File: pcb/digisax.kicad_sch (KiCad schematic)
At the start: 53 parts, among them SW1 RotaryEncoder_Switch, U1 ER_OLEDM0.91_1x-I2C, U2 MPXV7007, U3 MCP3221, U4 TLV320DAC3100_breakout, U5 ESP32-S3

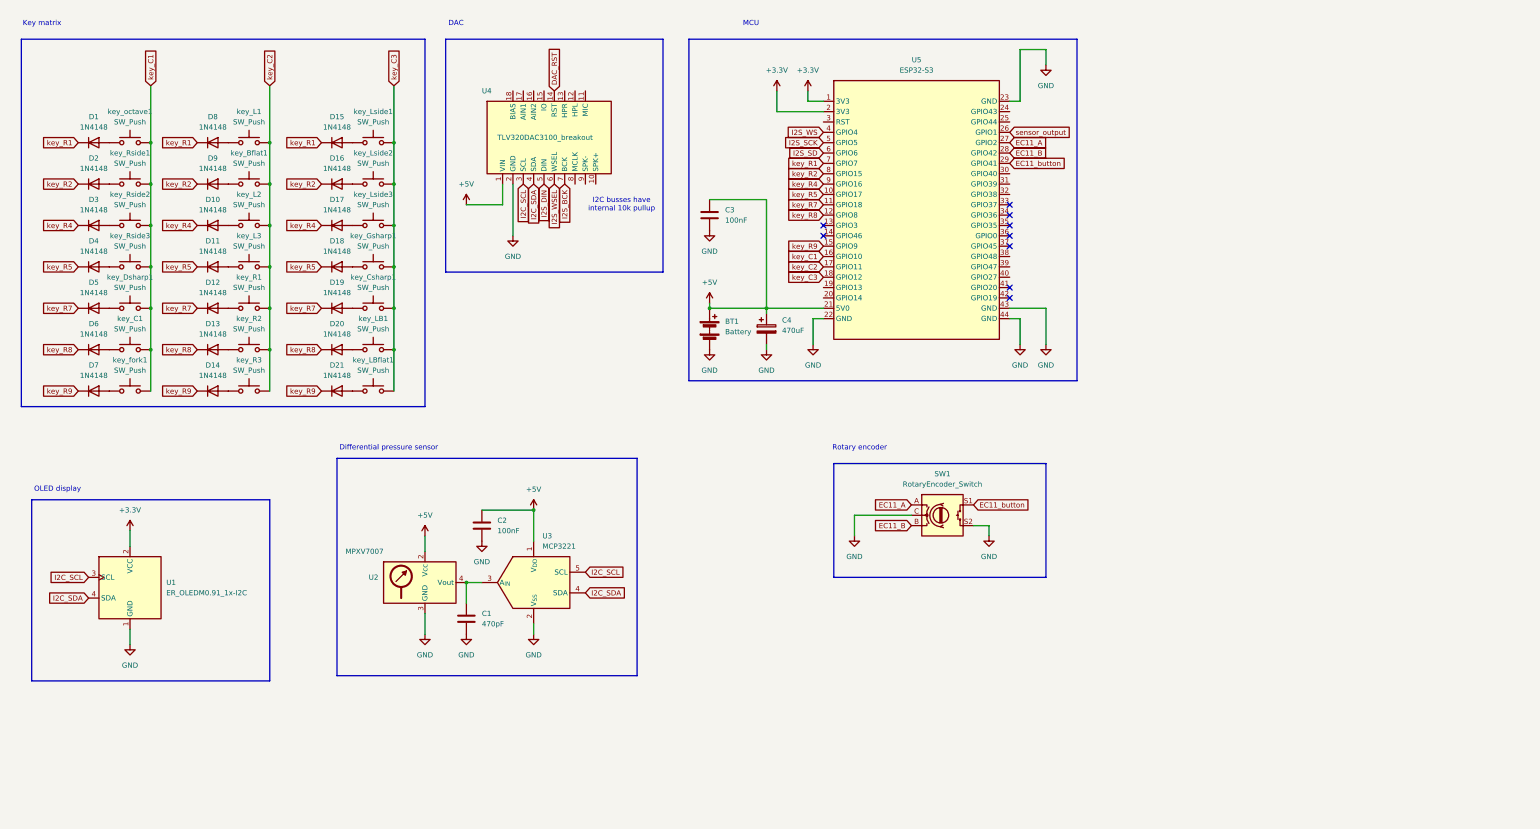
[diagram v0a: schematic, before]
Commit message: added headers to schem
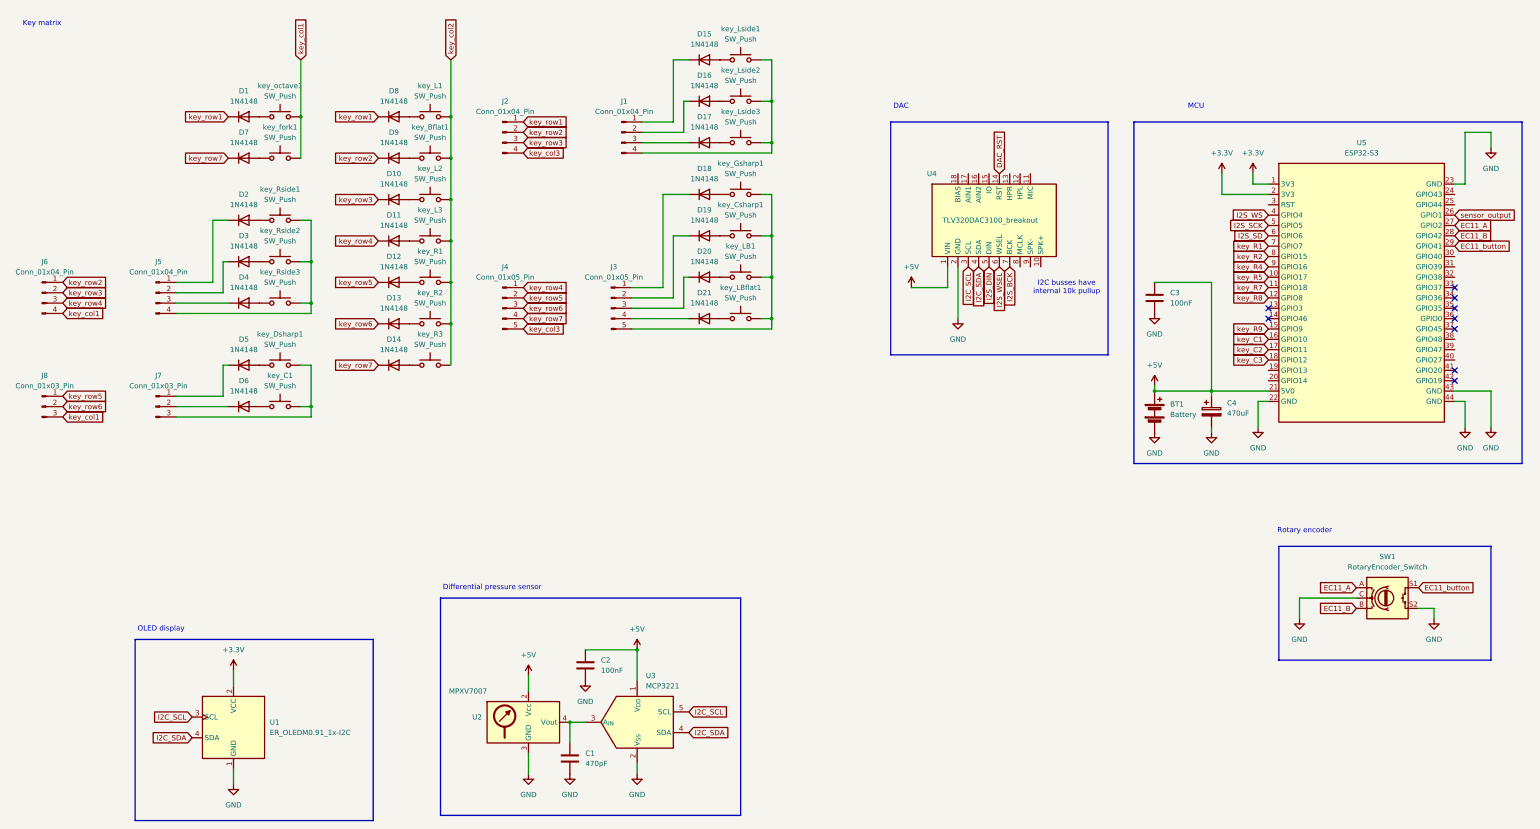
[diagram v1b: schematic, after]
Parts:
- added J1, J2, J5, J6: Conn_01x04_Pin, symbol Connector:Conn_01x04_Pin
- added J3, J4: Conn_01x05_Pin, symbol Connector:Conn_01x05_Pin
- added J7, J8: Conn_01x03_Pin, symbol Connector:Conn_01x03_Pin
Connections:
- net key_C1: no longer key_C1.2, key_Dsharp1.2, key_Rside1.2, key_Rside2.2, key_Rside3.2, key_fork1.2, key_octave1.2
- net key_C2: no longer key_Bflat1.2, key_L1.2, key_L2.2, key_L3.2, key_R1.2, key_R2.2, key_R3.2
- net key_C3: no longer key_Csharp1.2, key_Gsharp1.2, key_LB1.2, key_LBflat1.2, key_Lside1.2, key_Lside2.2, key_Lside3.2
- net key_R1: no longer D1.1 (K), D15.1 (K), D8.1 (K)
- net key_R2: no longer D16.1 (K), D2.1 (K), D9.1 (K)
- net key_R4: no longer D10.1 (K), D17.1 (K), D3.1 (K)
- net key_R5: no longer D11.1 (K), D18.1 (K), D4.1 (K)
- net key_R7: no longer D12.1 (K), D19.1 (K), D5.1 (K)
- net key_R8: no longer D13.1 (K), D20.1 (K), D6.1 (K)
- net key_R9: no longer D14.1 (K), D21.1 (K), D7.1 (K)
- new net: J1.4 (Pin_4), key_Lside1.2, key_Lside2.2, key_Lside3.2
- new net: J7.3 (Pin_3), key_C1.2, key_Dsharp1.2
- new net: D6.1 (K), J7.2 (Pin_2)
- new net: D15.1 (K), J1.1 (Pin_1)
- new net: D19.1 (K), J3.2 (Pin_2)
- new net: D4.1 (K), J5.3 (Pin_3)
- new net: J3.5 (Pin_5), key_Csharp1.2, key_Gsharp1.2, key_LB1.2, key_LBflat1.2
- new net: D2.1 (K), J5.1 (Pin_1)
- new net: J5.4 (Pin_4), key_Rside1.2, key_Rside2.2, key_Rside3.2
- new net: D3.1 (K), J5.2 (Pin_2)
- new net: D16.1 (K), J1.2 (Pin_2)
- new net: D18.1 (K), J3.1 (Pin_1)
- new net: D5.1 (K), J7.1 (Pin_1)
- new net: D17.1 (K), J1.3 (Pin_3)
- new net: D20.1 (K), J3.3 (Pin_3)
- new net: D21.1 (K), J3.4 (Pin_4)
- new net key_col1: J6.4 (Pin_4), J8.3 (Pin_3), key_fork1.2, key_octave1.2
- new net key_col2: key_Bflat1.2, key_L1.2, key_L2.2, key_L3.2, key_R1.2, key_R2.2, key_R3.2
- new net key_col3: J2.4 (Pin_4), J4.5 (Pin_5)
- new net key_row1: D1.1 (K), D8.1 (K), J2.1 (Pin_1)
- new net key_row2: D9.1 (K), J2.2 (Pin_2), J6.1 (Pin_1)
- new net key_row3: D10.1 (K), J2.3 (Pin_3), J6.2 (Pin_2)
- new net key_row4: D11.1 (K), J4.1 (Pin_1), J6.3 (Pin_3)
- new net key_row5: D12.1 (K), J4.2 (Pin_2), J8.1 (Pin_1)
- new net key_row6: D13.1 (K), J4.3 (Pin_3), J8.2 (Pin_2)
- new net key_row7: D14.1 (K), D7.1 (K), J4.4 (Pin_4)
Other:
- moved on the sheet: BT1, C1, C2, C3, C4, D1, D10, D11, D12, D13, D14, D15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

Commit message: more kcal burnt on pcb
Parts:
- J1, J2, J5, J6: footprint (none) -> digisax_stuff:pad_1x4
- J3, J4: footprint (none) -> digisax_stuff:pad_1x5
- J7, J8: footprint (none) -> digisax_stuff:pad_1x3
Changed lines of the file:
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@@
 			)
 		)
-		(property "Footprint" ""
+		(property "Footprint" "digisax_stuff:pad_1x4"
 			(at 24.13 90.17 0)
 			(hide yes)
@@
 			)
 		)
-		(property "Footprint" ""
+		(property "Footprint" "digisax_stuff:pad_1x3"
 			(at 24.13 118.11 0)
 			(hide yes)
@@
 			)
 		)
-		(property "Footprint" ""
+		(property "Footprint" "digisax_stuff:pad_1x4"
 			(at 52.07 90.17 0)
 			(hide yes)
@@
 			)
 		)
-		(property "Footprint" ""
+		(property "Footprint" "digisax_stuff:pad_1x5"
 			(at 137.16 93.98 0)
 			(hide yes)
@@
 			)
 		)
-		(property "Footprint" ""
+		(property "Footprint" "digisax_stuff:pad_1x3"
 			(at 52.07 118.11 0)
 			(hide yes)
@@
 			)
 		)
-		(property "Footprint" ""
+		(property "Footprint" "digisax_stuff:pad_1x4"
 			(at 166.37 50.8 0)
 			(hide yes)
@@
 			)
 		)
-		(property "Footprint" ""
+		(property "Footprint" "digisax_stuff:pad_1x5"
 			(at 163.83 93.98 0)
 			(hide yes)
@@
 			)
 		)
-		(property "Footprint" ""
+		(property "Footprint" "digisax_stuff:pad_1x4"
 			(at 137.16 50.8 0)
 			(hide yes)
